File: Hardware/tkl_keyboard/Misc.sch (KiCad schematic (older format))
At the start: 16 parts, among them J6 Conn_01x04_Female, SW90 Rotary_Encoder_Switch, SW91 Rotary_Encoder_Switch, SW92 Rotary_Encoder_Switch

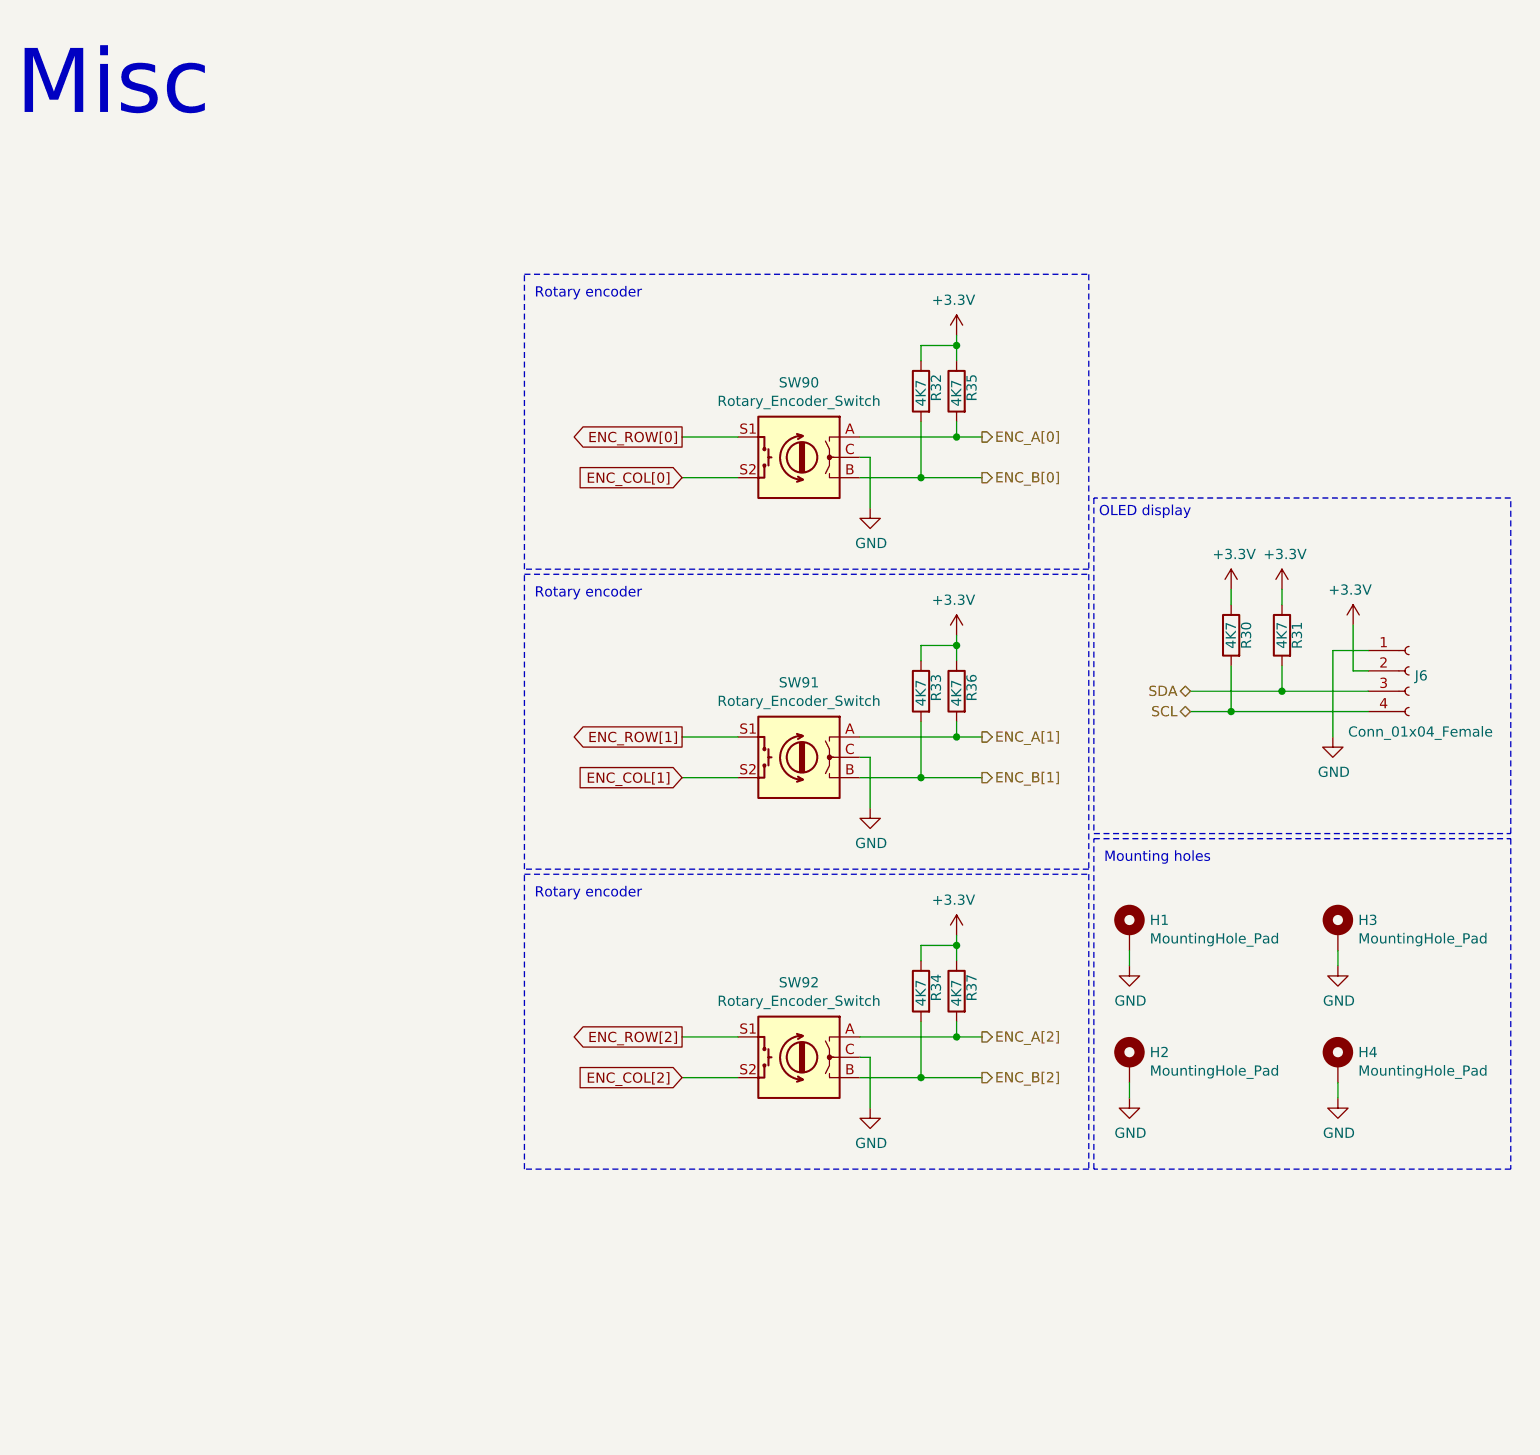
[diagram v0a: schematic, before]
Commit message: Updating schematic
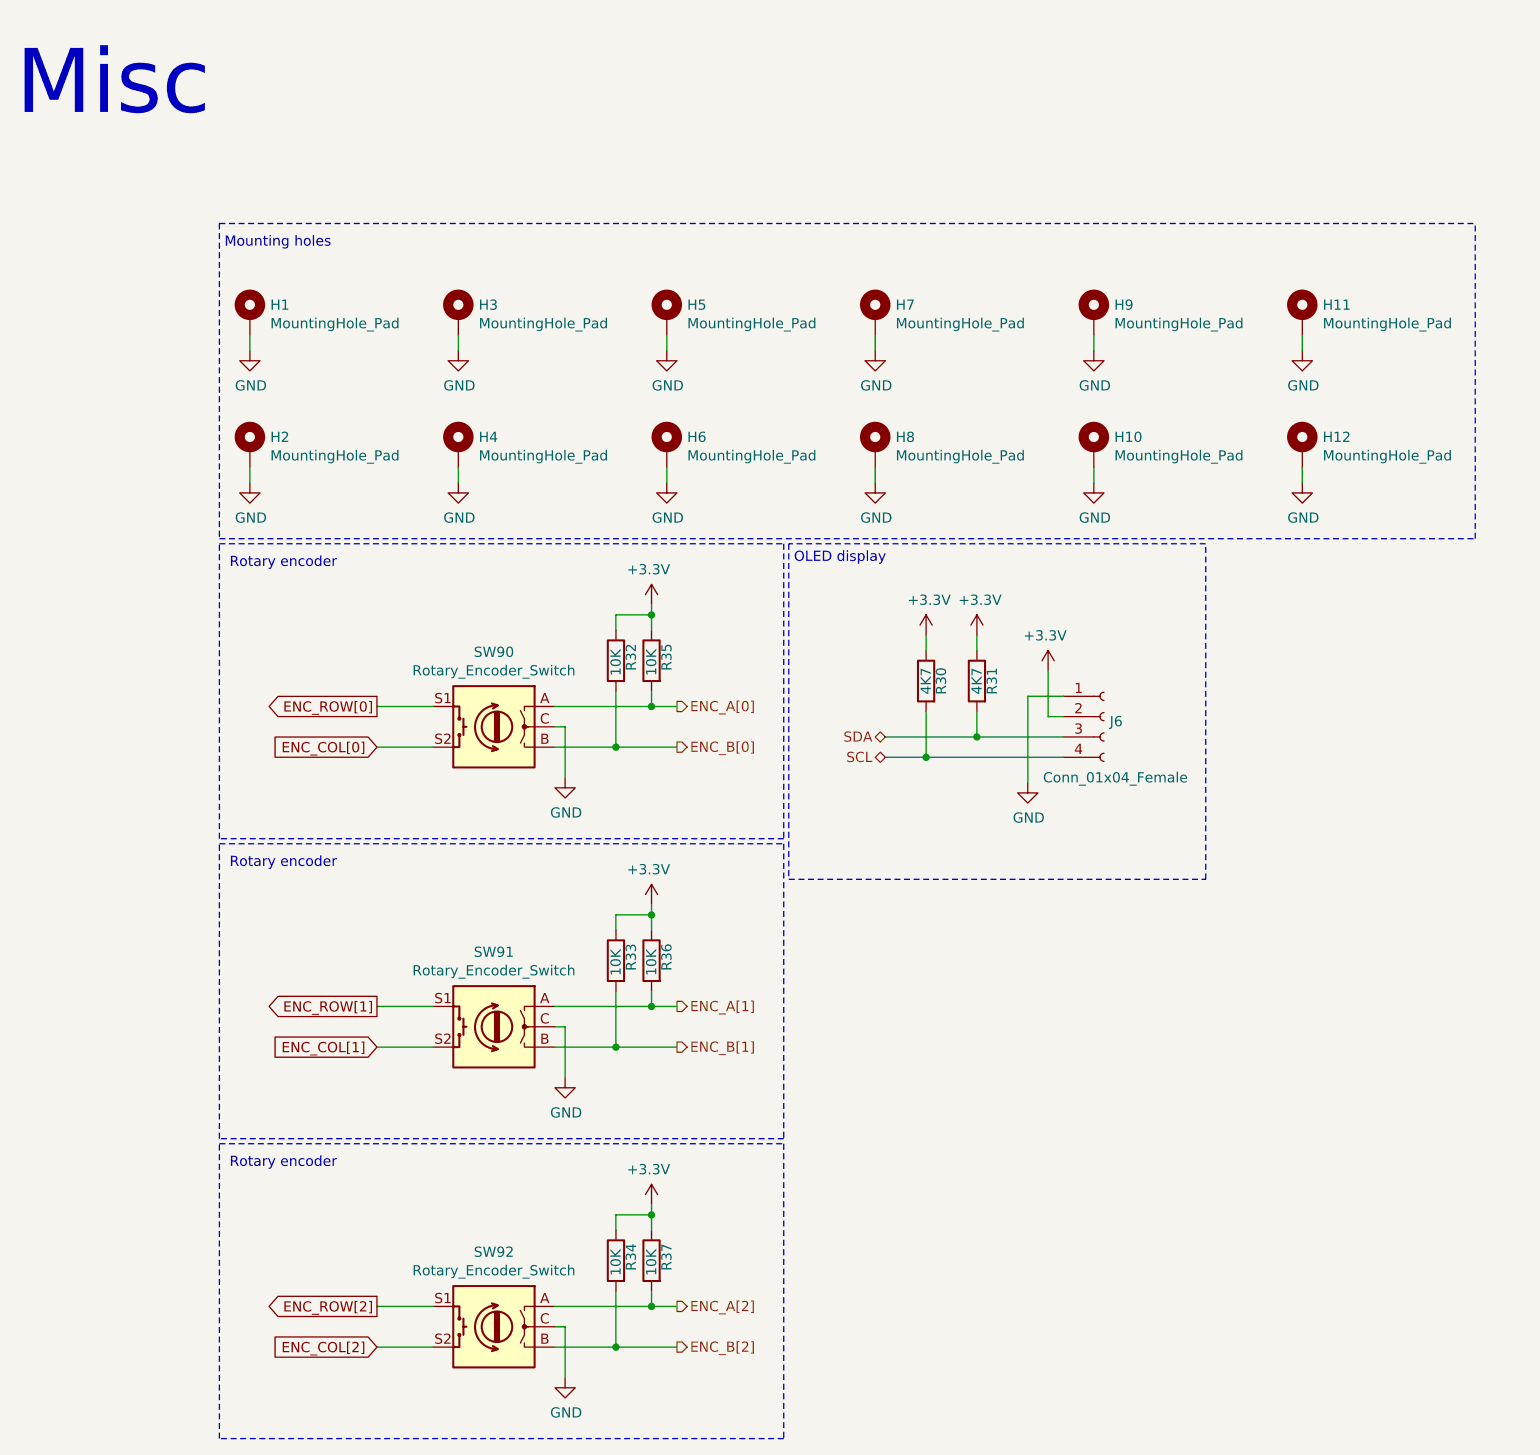
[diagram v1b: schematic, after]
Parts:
- added H10, H11, H12, H5, H6, H7, H8, H9: MountingHole_Pad, mounting_hole:MountingHole_3.2mm_M3_ISO7380_Pad, symbol Mechanical:MountingHole_Pad
- R32, R33, R34, R35, R36, R37: value 4K7 -> 10K
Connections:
- net GND: now also H10.1, H11.1, H12.1, H5.1, H6.1, H7.1, H8.1, H9.1
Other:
- moved on the sheet: H1, H2, H3, H4, J6, R30, R31, R32, R33, R34, R35, R36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
